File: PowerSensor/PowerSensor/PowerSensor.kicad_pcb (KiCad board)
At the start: 2 copper layers, 35.6 x 22.6 mm, 12 parts, among them J1 Current Sens, J3 BAT+, J4 BAT-, J5 Screw_Terminal_01x04, U1 ACS712ELCTR-20A-T_NRND

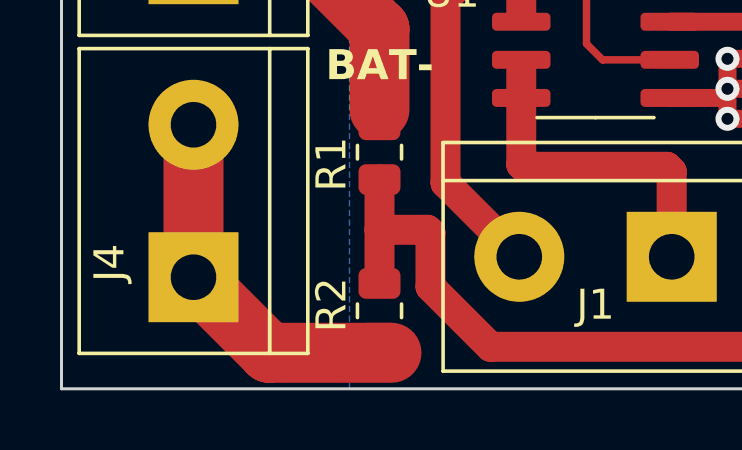
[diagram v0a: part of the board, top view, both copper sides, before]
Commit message: PCB optimozation
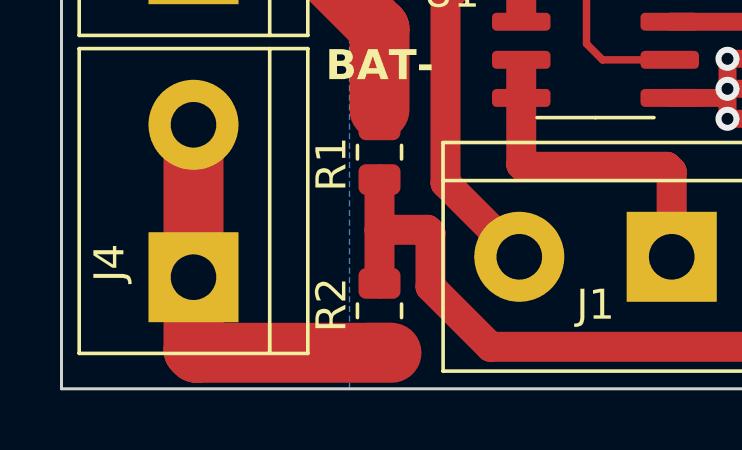
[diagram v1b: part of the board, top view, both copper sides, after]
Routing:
- net Battery(-): track 12.7 -> 14.1 mm
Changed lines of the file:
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@@
   (segment (start 104.2 96.94) (end 104.2 90.8) (width 1) (layer "F.Cu") (net 4))
   (segment (start 106.725 90.295) (end 106.725 91.3) (width 1) (layer "F.Cu") (net 4))
-  (segment (start 102.4 102.6) (end 98.32 102.6) (width 2) (layer "F.Cu") (net 5))
+  (segment (start 95.9 102.6) (end 95.8 102.5) (width 2) (layer "F.Cu") (net 5))
+  (segment (start 102.4 102.6) (end 95.9 102.6) (width 2) (layer "F.Cu") (net 5))
   (segment (start 95.8 95) (end 95.8 100.08) (width 2) (layer "F.Cu") (net 5))
-  (segment (start 98.32 102.6) (end 95.8 100.08) (width 2) (layer "F.Cu") (net 5))
+  (segment (start 95.8 102.5) (end 95.8 100.08) (width 2) (layer "F.Cu") (net 5))
   (segment (start 109.8 90) (end 110.095 90.295) (width 0.25) (layer "F.Cu") (net 6))
   (segment (start 115.04 89.44) (end 113.3 87.7) (width 0.25) (layer "F.Cu") (net 6))
